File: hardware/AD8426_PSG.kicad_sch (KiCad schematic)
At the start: 19 parts, among them U4 AD8426BCPZ-WP

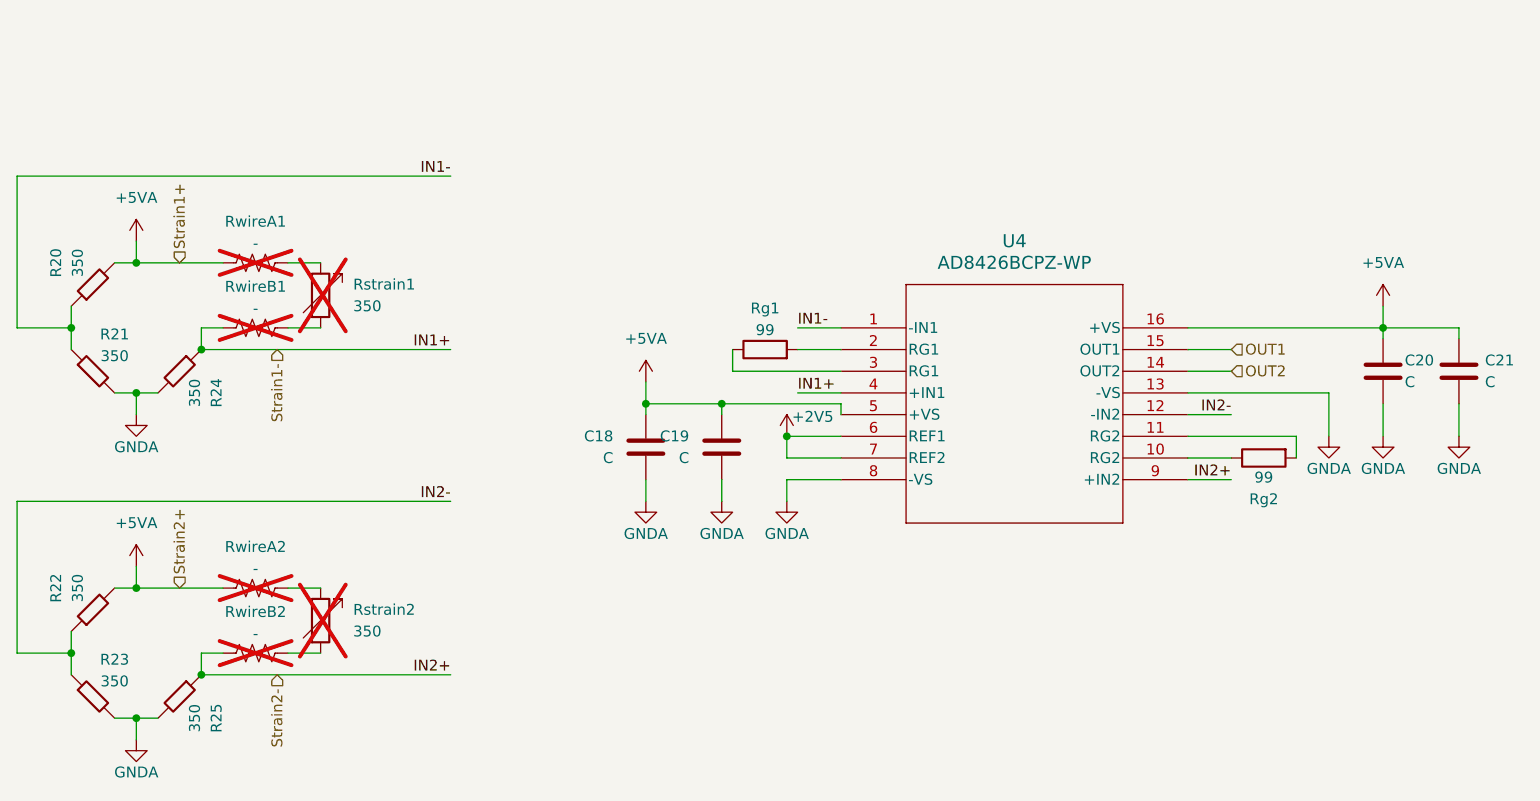
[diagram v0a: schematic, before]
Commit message: updated some docs
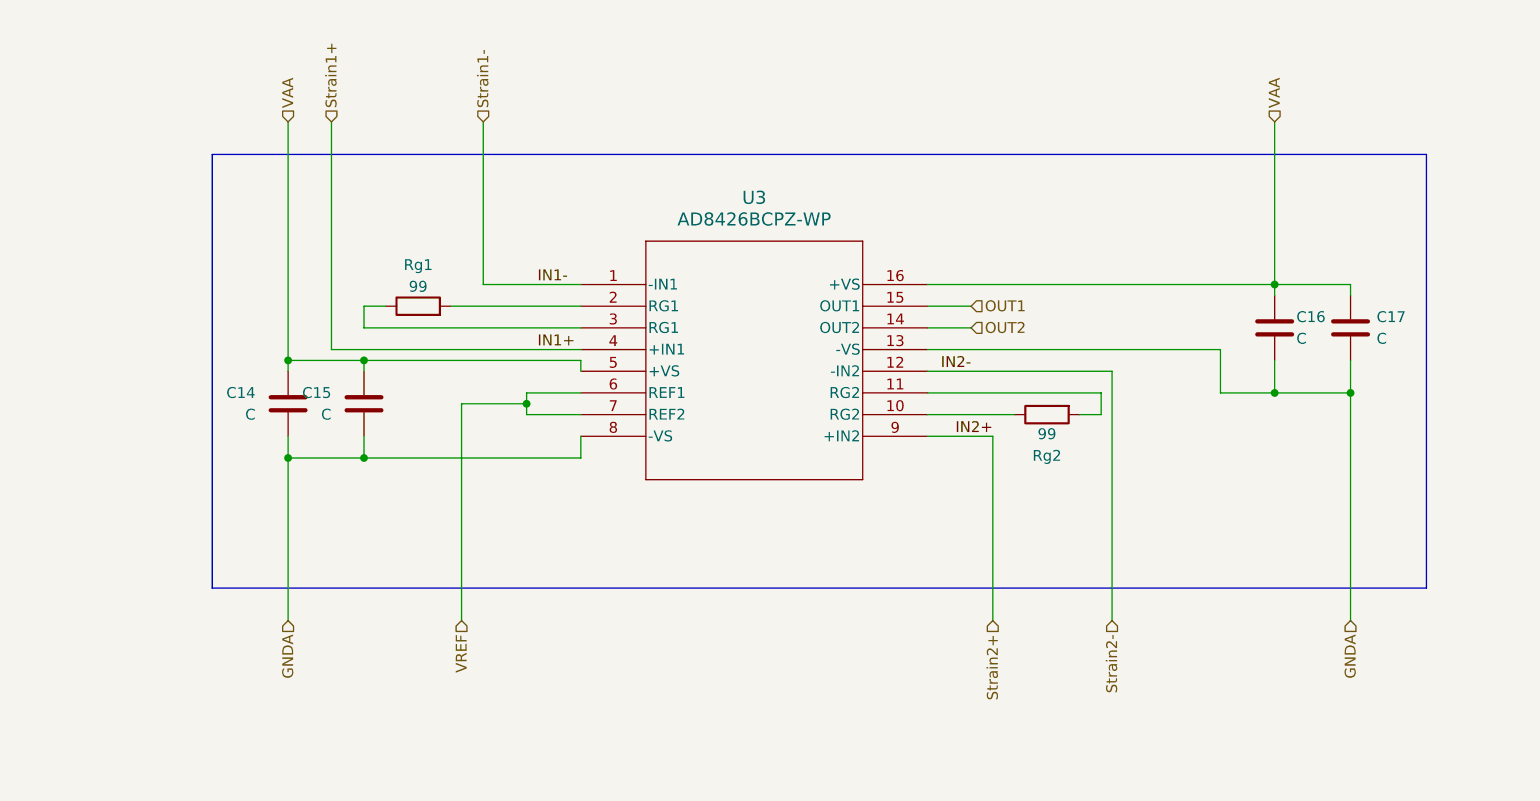
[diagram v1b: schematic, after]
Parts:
- removed R20, R21, R22, R23, R24, R25: 350, symbol Device:R_45deg
- removed Rstrain1, Rstrain2: 350, symbol Device:R_Variable
- removed RwireA1, RwireA2, RwireB1, RwireB2: -, symbol Device:R_US
- renumbered C18 to C14, C19 to C15, C20 to C16, C21 to C17, U4 to U3
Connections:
- net IN1- is gone; now on net Strain1-: U3.1 (-IN1)
- net IN2- is gone; now on net Strain2-: U3.12 (-IN2)
- net Strain1-: no longer U3.4 (+IN1)
- net Strain2-: no longer U3.9 (+IN2)
- net +2V5 renamed VREF
- net +5VA renamed VAA
- new net Strain1+: U3.4 (+IN1)
- new net Strain2+: U3.9 (+IN2)
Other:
- moved on the sheet: C14, C15, C16, C17, Rg1, Rg2, U3
